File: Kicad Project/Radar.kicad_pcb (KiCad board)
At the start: 2 copper layers, 30 parts

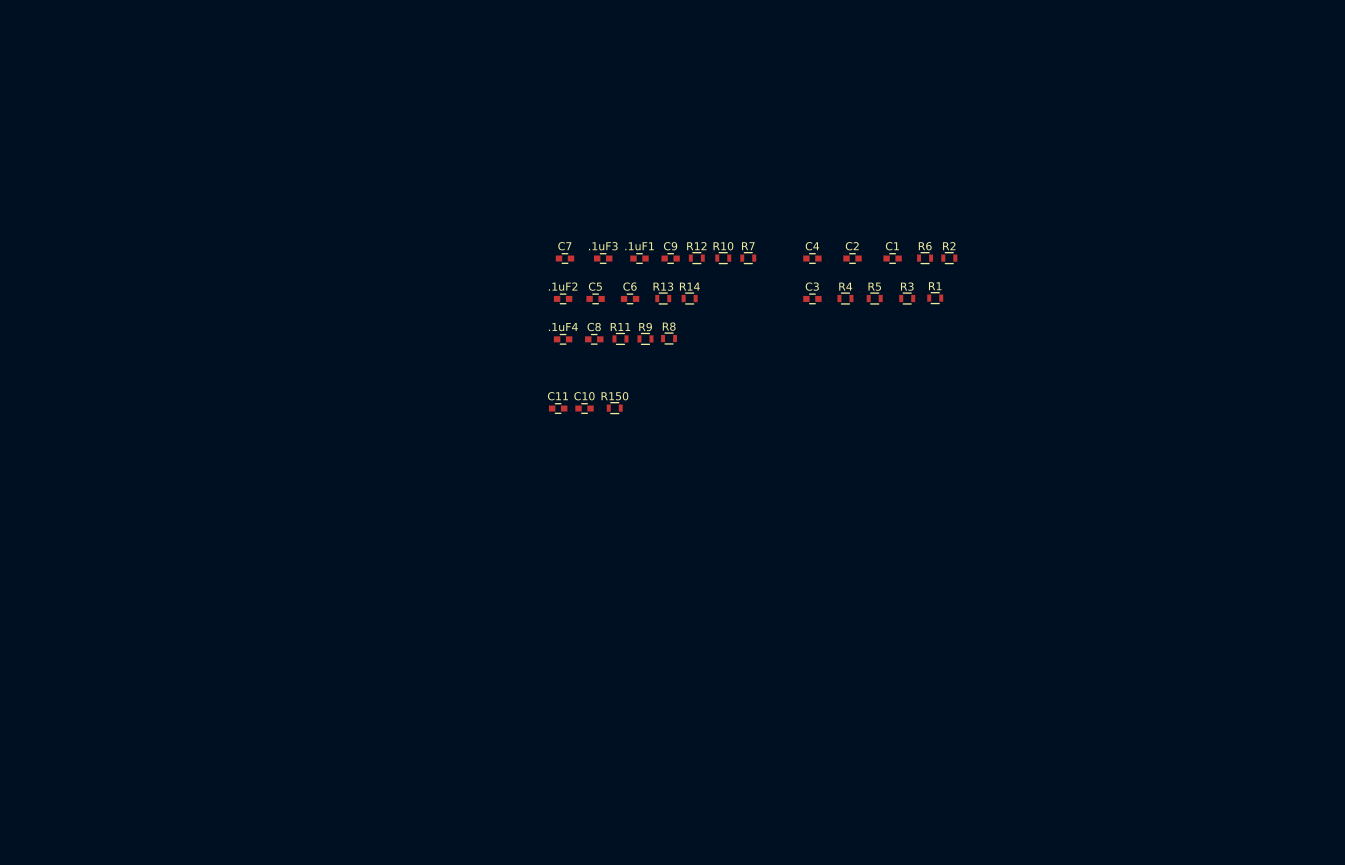
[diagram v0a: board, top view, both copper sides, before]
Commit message: PCB Changes
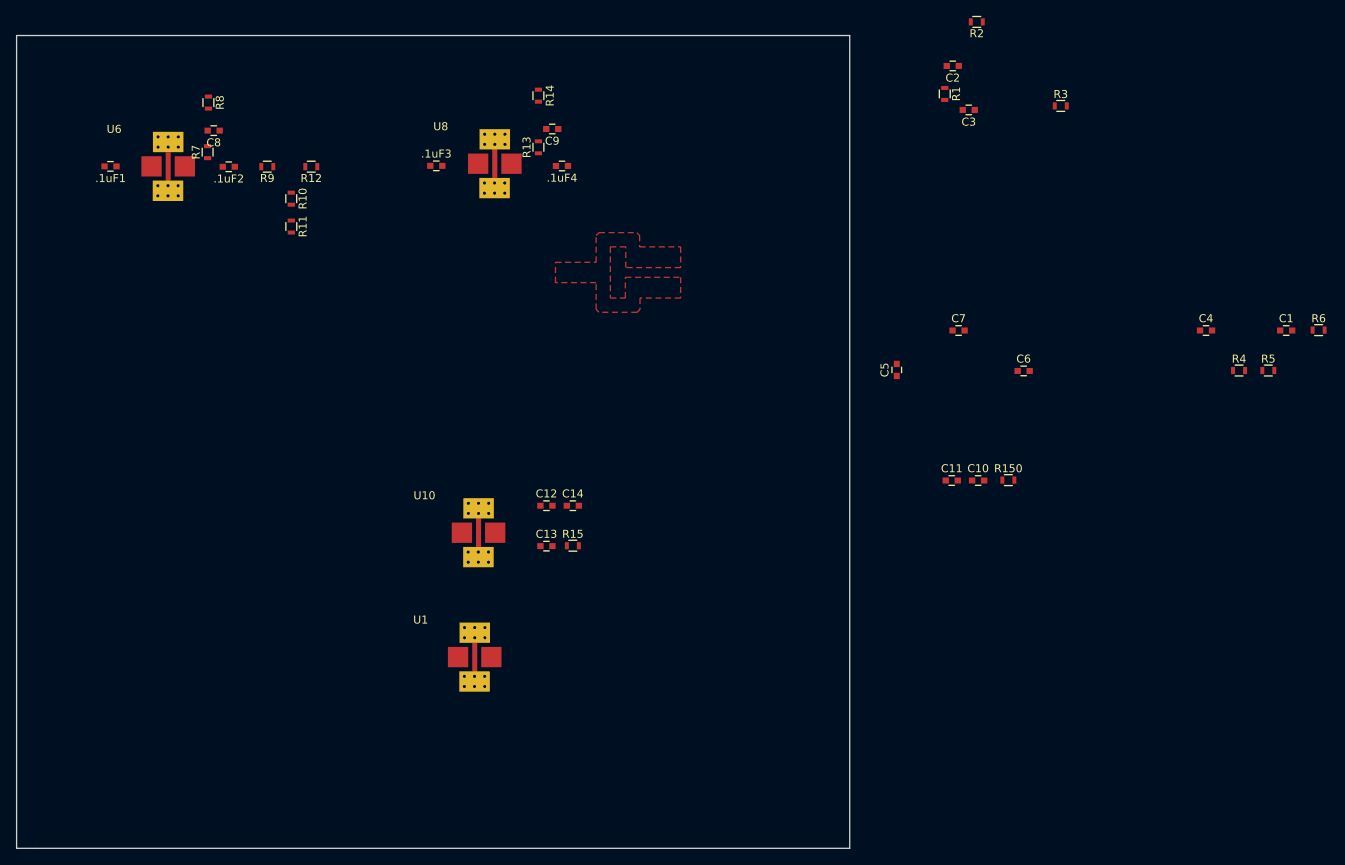
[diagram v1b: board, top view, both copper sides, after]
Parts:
- added C12: C, Capacitors_SMD:C_0603, F.Cu at (160.2, 135.0)
- added C13: C, Capacitors_SMD:C_0603, F.Cu at (160.2, 140.0)
- added C14: C, Capacitors_SMD:C_0603, F.Cu at (163.5, 135.0)
- added R15: R, Resistors_SMD:R_0603, F.Cu at (163.5, 140.0)
- added U1: GALI-1+, RadarComponents:Amplifier, F.Cu at (150.4, 155.2)
- added U10: GALI-2+, RadarComponents:Amplifier, F.Cu at (150.9, 139.6)
- added U6: GALI-2+, RadarComponents:Amplifier, F.Cu at (112.1, 93.8)
- added U8: GALI-2+, RadarComponents:Amplifier, F.Cu at (152.9, 93.5)
- moved R7 68.9 mm to (117.9, 90.8), turned to 90 degrees
- moved .1uF1 67.1 mm to (105.7, 92.6), turned to 180 degrees
- moved R8 64.7 mm to (118.0, 84.6), turned to 270 degrees
- moved R10 54.5 mm to (128.3, 96.6), turned to 270 degrees
- moved C8 54.3 mm to (118.6, 88.1), turned to 180 degrees
- moved R9 51.9 mm to (125.3, 92.6), turned to 180 degrees
- moved C4 50.0 mm to (242.7, 113.1)
- moved R6 50.0 mm to (256.7, 113.0)
- moved C1 50.0 mm to (252.7, 113.1)
- moved C6 50.0 mm to (219.9, 118.1)
- moved C7 50.0 mm to (211.7, 113.1)
- moved R150 50.0 mm to (217.9, 131.8)
- moved R4 50.0 mm to (246.8, 118.1)
- moved R5 50.0 mm to (250.4, 118.1)
- moved C10 50.0 mm to (214.2, 131.8)
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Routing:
- added copper zone on F.Cu, net (none)
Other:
- board outline added: 104.1 x 101.6 mm

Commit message: PCB and Schematic updates
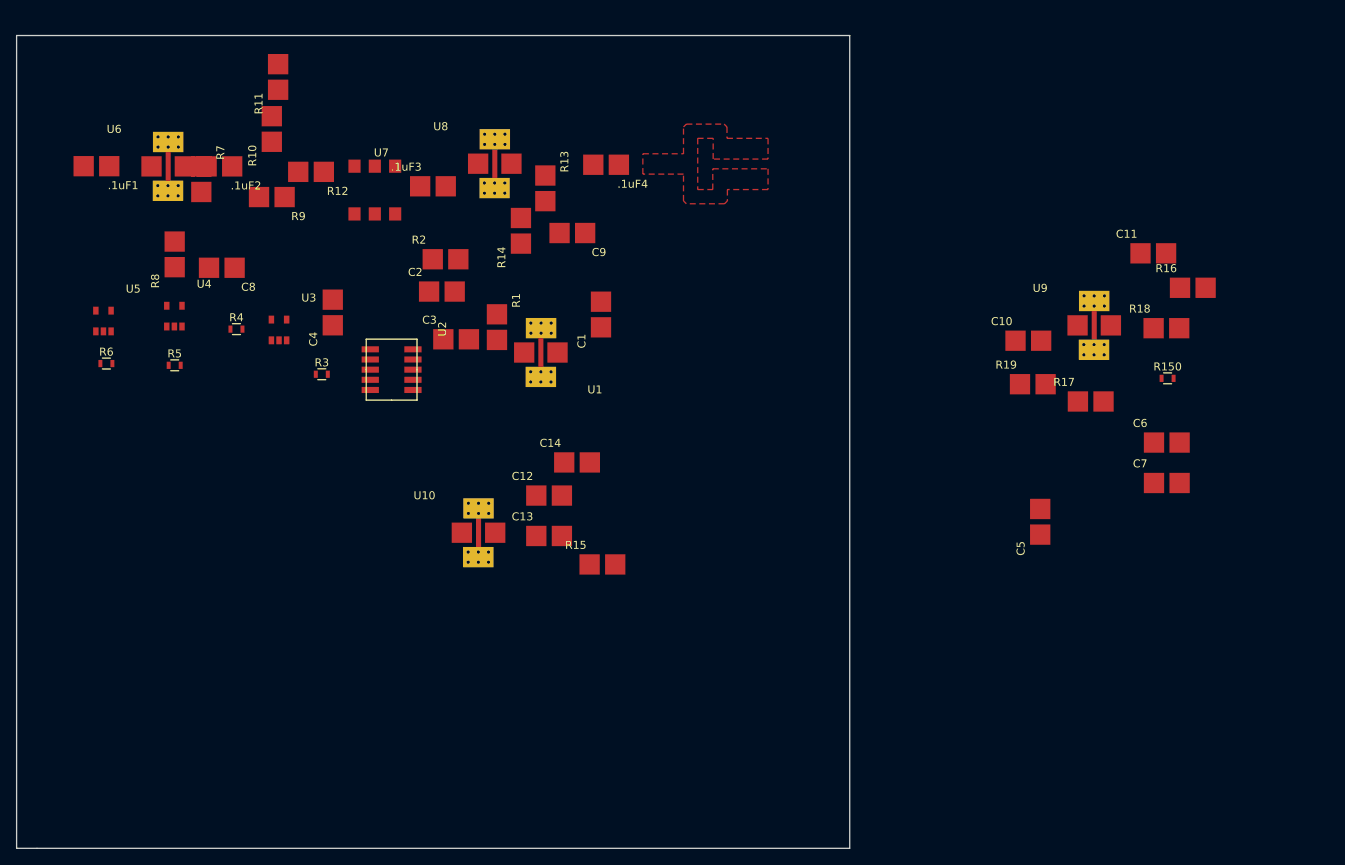
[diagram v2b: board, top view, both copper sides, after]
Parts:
- added R16: 75, RadarComponents:100PAD, F.Cu at (240.7, 109.0)
- added R17: 75, RadarComponents:100PAD, F.Cu at (227.9, 123.2)
- added R18: 75, RadarComponents:100PAD, F.Cu at (237.4, 114.1)
- added R19: 75, RadarComponents:100PAD, F.Cu at (220.7, 121.1)
- added U2: MCA1-85L+, RadarComponents:DZ885, F.Cu at (140.9, 118.0)
- added U3: LMV751, RadarComponents:SOT23-5, F.Cu at (125.8, 112.8)
- added U4: LMV751, RadarComponents:SOT23-5, F.Cu at (112.8, 111.1)
- added U5: LMV751, RadarComponents:SOT23-5, F.Cu at (103.9, 111.7)
- added U7: RMK-3-93+, RadarComponents:TT1224, F.Cu at (135.4, 93.4)
- added U9: LEE-39+, RadarComponents:Amplifier, F.Cu at (227.9, 113.7)
- .1uF1, .1uF2, .1uF3, .1uF4, C1, C10, C11, C12, C13, C14, C2, C3, C4, C5, C6, C7, C8, C9: footprint Capacitors_SMD:C_0603 -> RadarComponents:100PAD
- R1, R10, R11, R12, R13, R14, R15, R2, R7, R8, R9: footprint Resistors_SMD:R_0603 -> RadarComponents:100PAD
- moved R6 151.6 mm to (105.2, 117.2)
- moved R5 136.7 mm to (113.7, 117.4)
- moved R4 125.4 mm to (121.5, 112.9)
- moved C4 107.9 mm to (134.8, 111.2), turned to 90 degrees
- moved R3 98.3 mm to (132.1, 118.5)
- moved C1 84.4 mm to (168.3, 111.4), turned to 90 degrees
- moved R2 73.6 mm to (147.3, 105.4), turned to 0 degrees
- moved C3 71.0 mm to (148.6, 115.4), turned to 0 degrees
- moved C2 70.6 mm to (146.8, 109.5), turned to 0 degrees
- moved R1 64.1 mm to (152.8, 112.3)
- moved U1 41.8 mm to (160.3, 114.6), turned to 180 degrees
- moved C11 36.8 mm to (235.7, 104.7)
- moved C7 32.8 mm to (237.4, 133.4)
- moved C5 27.2 mm to (223.2, 137.3)
- moved R150 23.6 mm to (237.9, 119.1)
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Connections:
- net Net-(.1uF4-Pad1) renamed /SourceModule.sch/PowerSplitter
- net Net-(C10-Pad2) renamed /TXRX Module/receive_out
- net Net-(C11-Pad2) renamed /TXRX Module/transmit_in
- C12 pad 1: Net-(C12-Pad1) -> GND
- C13 pad 2: Net-(C13-Pad2) -> GND
- R1 pad 2: Net-(R1-Pad2) -> Net-(C3-Pad2)
- U10 pad 1: Net-(U10-Pad1) -> Net-(C11-Pad1)
- U10 pad 2: Net-(U10-Pad2) -> GND
- U10 pad 3: Net-(U10-Pad3) -> Net-(C14-Pad2)
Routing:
- added copper zone on F.Cu, net /SourceModule.sch/PowerSplitter
- removed copper zone on F.Cu, net (none)
